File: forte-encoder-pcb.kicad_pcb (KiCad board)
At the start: 6 copper layers, 36.5 x 45 mm, 54 parts, among them J1 Conn_01x01_Pin, J10 Conn_01x01_Pin, J2 BM07B-GHS-TBT, J4 Conn_01x01_Pin, J7 Conn_01x01_Pin, J8 Conn_01x01_Pin, J9 Conn_01x01_Pin, U2 STM32F103C8Tx, U3 MCP2542FD-E/MF, U4 MA732GQ-Z, U5 TPS629203DRLR, U6 TPS629203DRLR, Y1 CSTNE8M00G550000R0

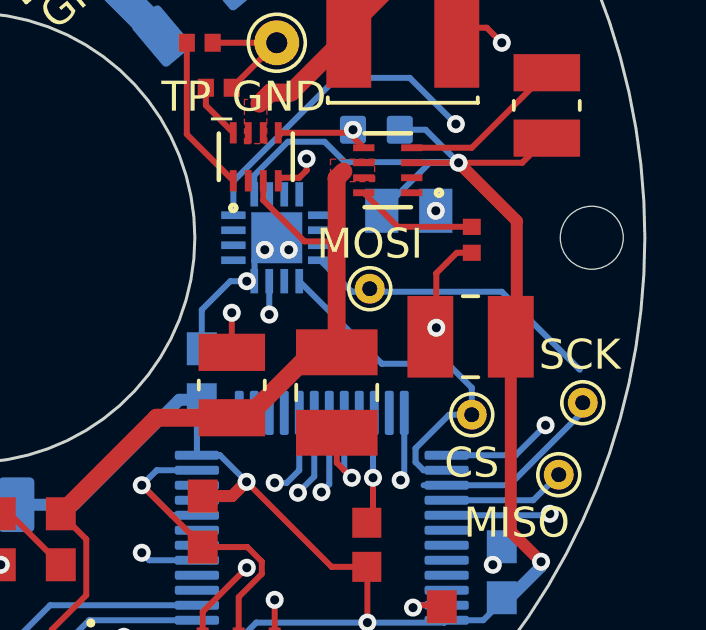
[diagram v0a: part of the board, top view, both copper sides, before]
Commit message: tiiny fix
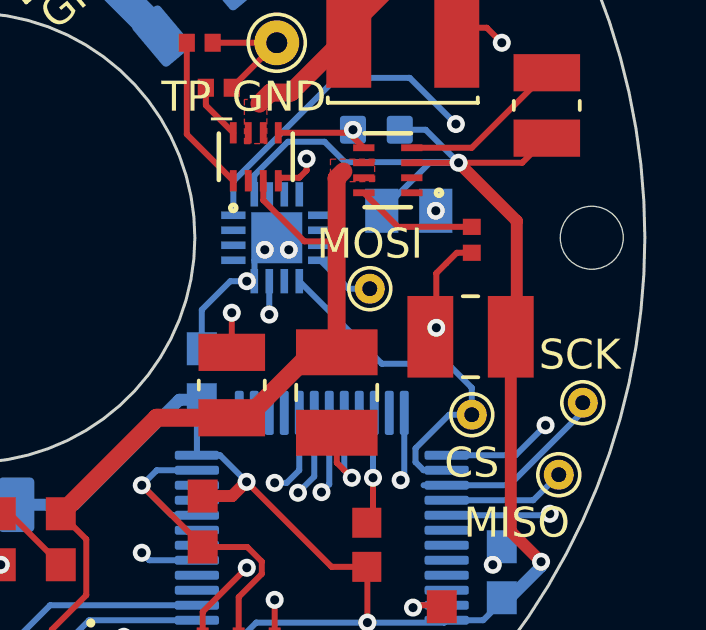
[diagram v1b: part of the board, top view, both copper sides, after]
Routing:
- net /MOSI: track 24.3 -> 16.1 mm
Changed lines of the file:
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@@
 	(segment
 		(start 107.4478 100.750001)
-		(end 108.497799 101.8)
+		(end 108.397799 101.7)
+		(width 0.2)
+		(layer "B.Cu")
+		(net "/MOSI")
+	)
+	(segment
+		(start 108.397799 101.7)
+		(end 109.1 101.7)
 		(width 0.2)
 		(layer "B.Cu")
@@
 	)
 	(segment
-		(start 108.497799 101.8)
-		(end 113.5 101.8)
-		(width 0.2)
-		(layer "B.Cu")
-		(net "/MOSI")
-	)
-	(segment
 		(start 115.1 109.2)
 		(end 115.05 109.25)
 		(width 0.2)
 		(layer "B.Cu")
-		(net "/MOSI")
-	)
-	(segment
-		(start 113.5 101.8)
-		(end 116.1 104.4)
-		(width 0.2)
-		(layer "B.Cu")
